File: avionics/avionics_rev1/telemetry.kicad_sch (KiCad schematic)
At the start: 11 parts, among them U11 MAX-M10S-00B

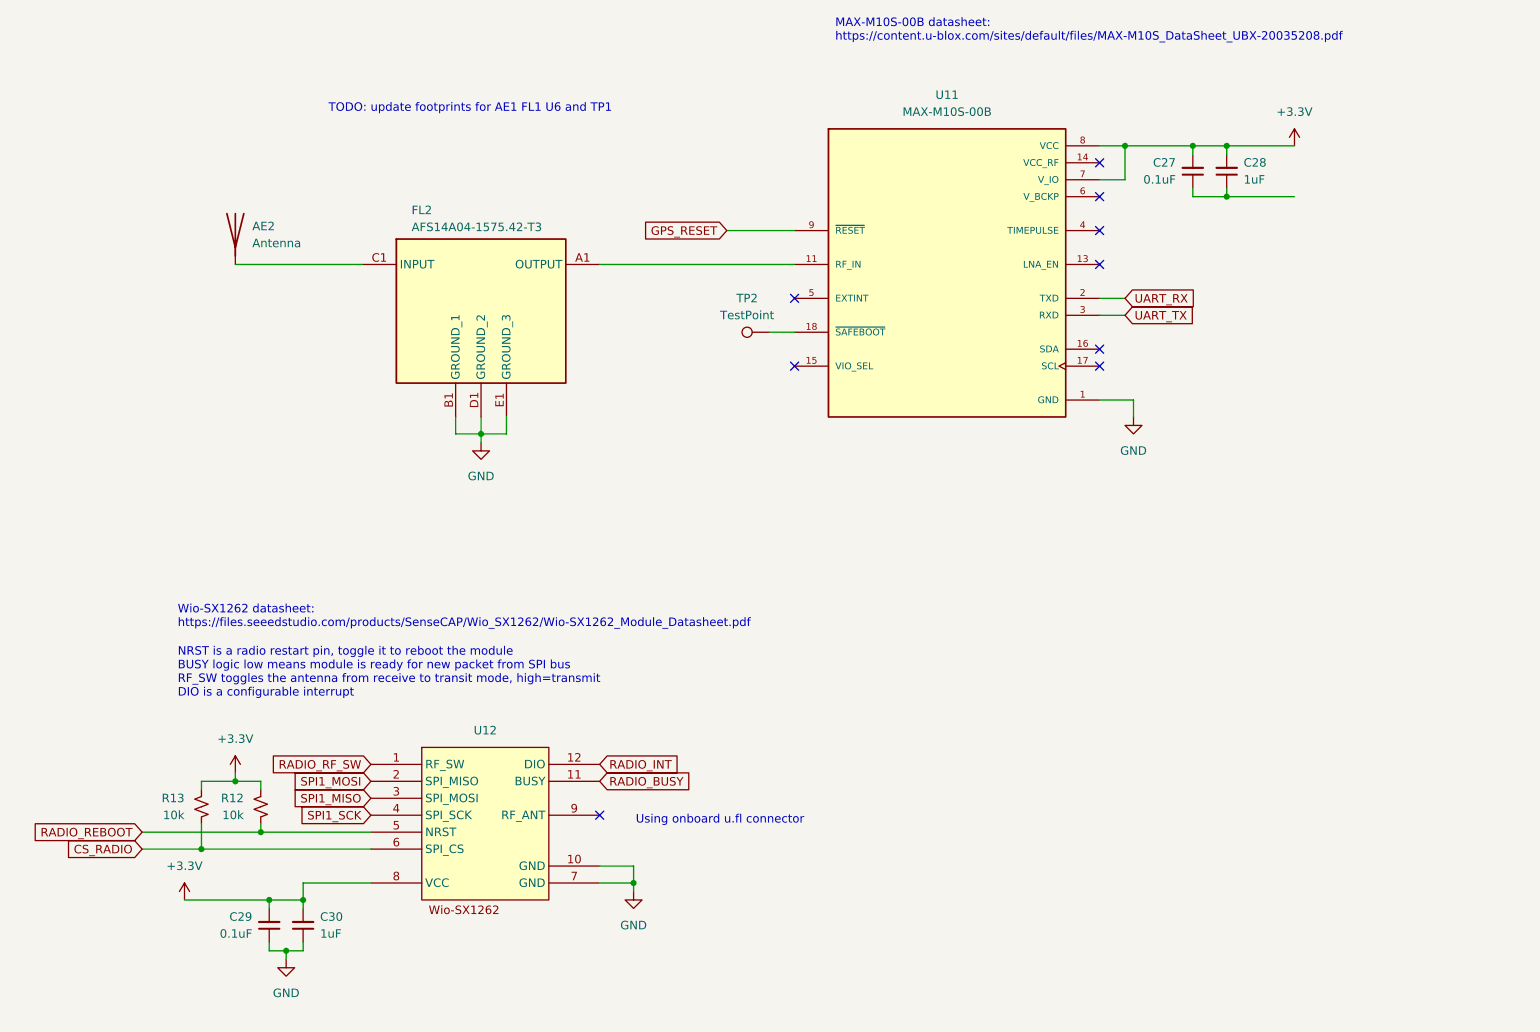
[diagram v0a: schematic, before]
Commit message: latest work
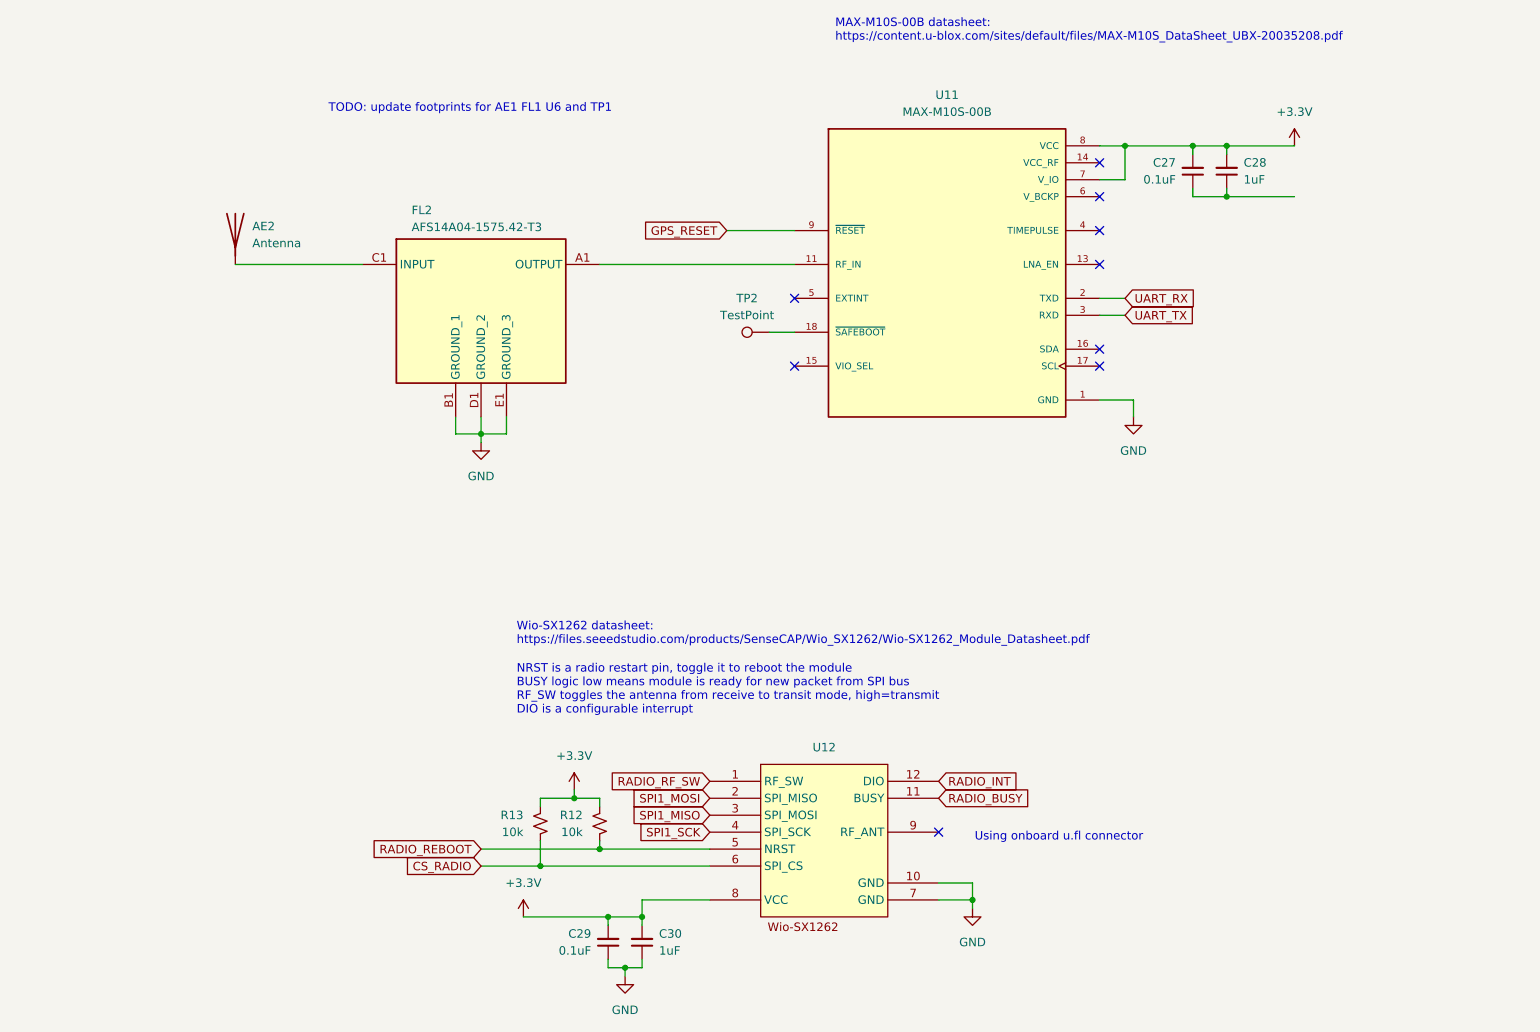
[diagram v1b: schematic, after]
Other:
- moved on the sheet: C29, C30, R12, R13, U12

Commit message: saving work before chat
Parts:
- U11: footprint avionics_footprints:XCVR_MAX-M10S-00B -> MAX-M10S-00B:XCVR_MAX-M10S-00B
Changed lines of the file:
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@@
 			)
 		)
-		(property "Footprint" "avionics_footprints:XCVR_MAX-M10S-00B"
+		(property "Footprint" "MAX-M10S-00B:XCVR_MAX-M10S-00B"
 			(at 153.162 38.354 0)
 			(hide yes)
